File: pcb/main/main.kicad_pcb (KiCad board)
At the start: 2 copper layers, 77.5 x 78.7 mm, 43 parts, among them J1 USB_B, J2 USB_B, J3 RJ45, J4 RJ45, J5 STLink, J6 XH6, J7 Conn_01x05, J8 COLS, SW1 RST_SW, SW2 IS_LEFT, SW3 IS_LEFT, SW4 BOOT0_SW, SW5 BOOT1_SW, U1 LM1117-3.3, U2 STM32F103C8Tx, Y1 8MHz, Y2 32.768

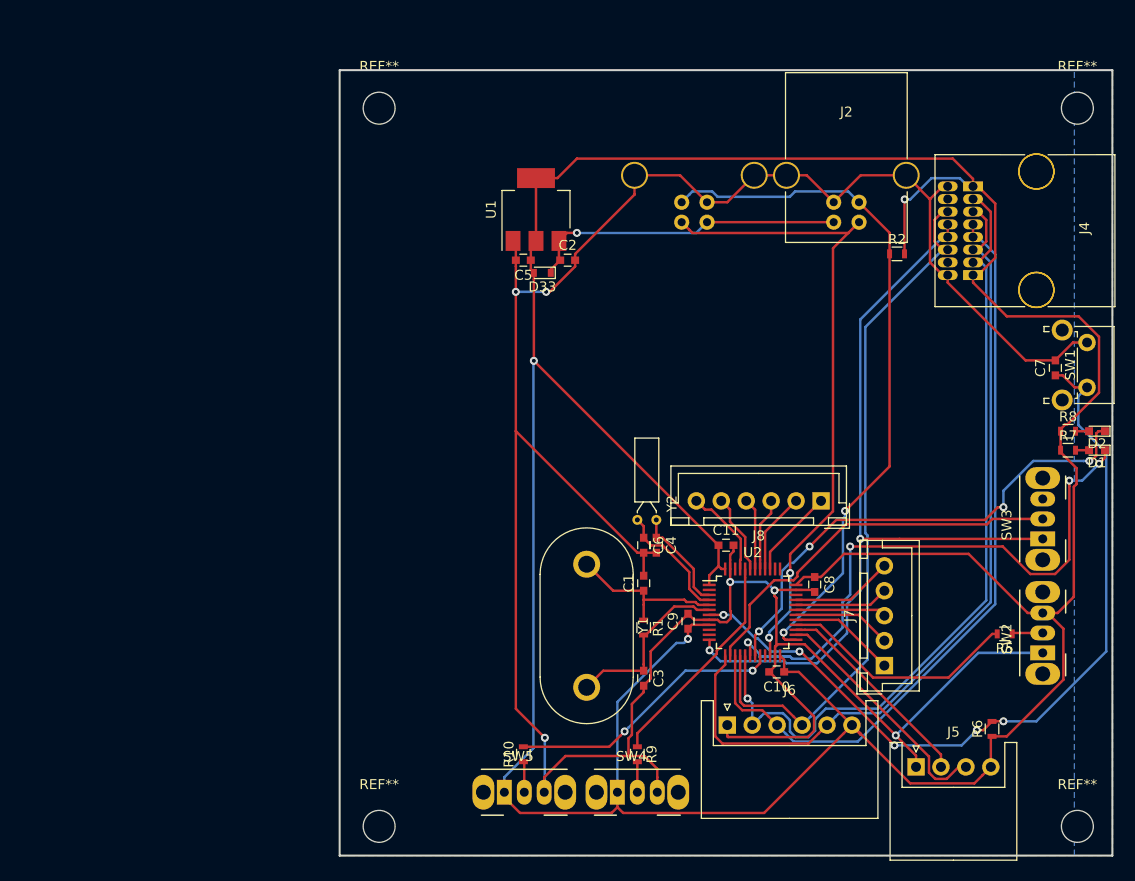
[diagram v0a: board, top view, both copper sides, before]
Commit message: fix main pcb
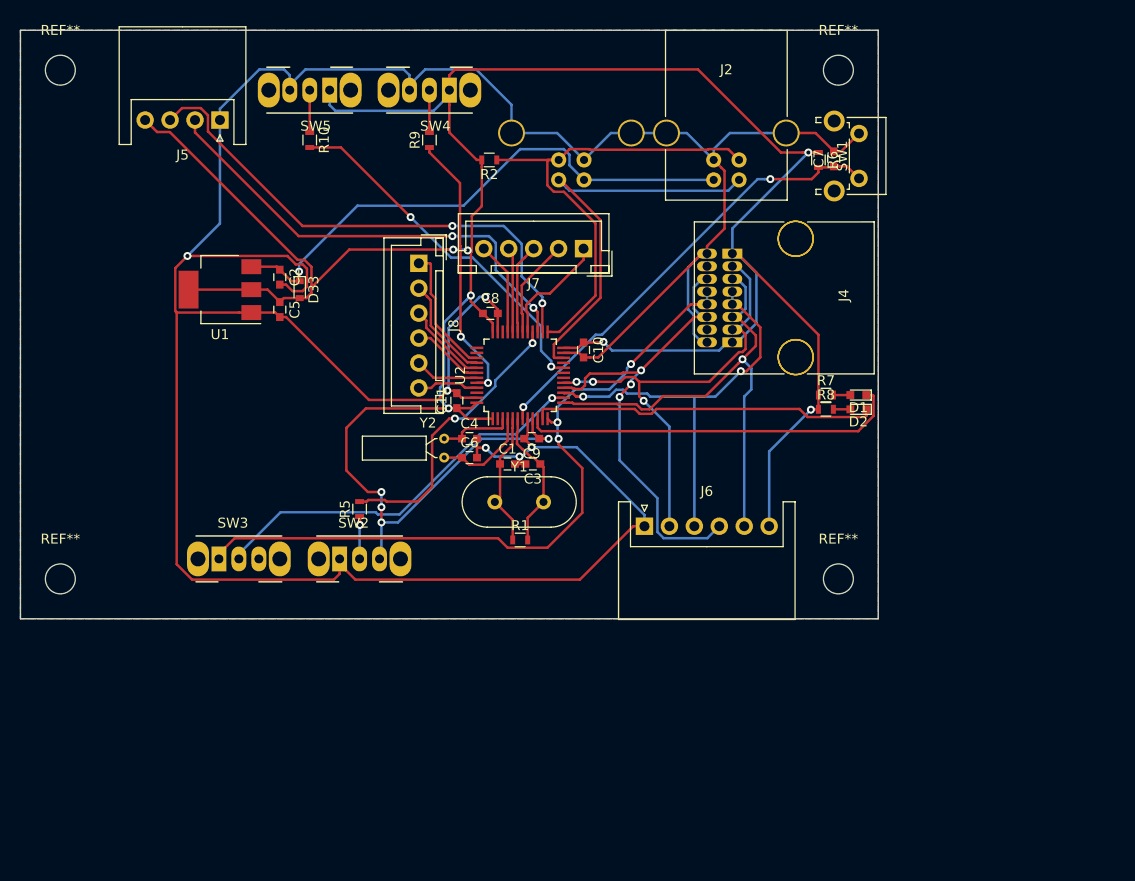
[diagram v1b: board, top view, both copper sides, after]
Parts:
- removed the REF** at (3.96, 3.81)
- removed the REF** at (74.0, 3.81)
- removed the REF** at (3.96, 75.8)
- removed the REF** at (74.0, 75.8)
- added REF**: MountingHole_3mm, Mounting_Holes:MountingHole_3mm, F.Cu at (-28.0, 0.00)
- added REF**: MountingHole_3mm, Mounting_Holes:MountingHole_3mm, F.Cu at (-28.0, 51.0)
- added REF**: MountingHole_3mm, Mounting_Holes:MountingHole_3mm, F.Cu at (50.0, 51.0)
- added REF**: MountingHole_3mm, Mounting_Holes:MountingHole_3mm, F.Cu at (50.0, 0.00)
- Y1: footprint Crystals:Crystal_HC33-U_Vertical -> Crystals:Crystal_HC49-4H_Vertical
- moved J5 95.3 mm to (-12.0, 5.00), turned to 180 degrees
- moved SW3 82.6 mm to (-12.1, 49.0), turned to 0 degrees
- moved SW5 72.5 mm to (-1.00, 2.00), turned to 180 degrees
- moved SW4 72.4 mm to (11.0, 2.00), turned to 180 degrees
- moved SW2 71.1 mm to (0.00, 49.0), turned to 0 degrees
- moved R5 65.9 mm to (2.00, 44.0), turned to 90 degrees
- moved R10 65.2 mm to (-3.00, 7.00), turned to 270 degrees
- moved R9 65.0 mm to (9.00, 7.00), turned to 90 degrees
- moved R6 59.6 mm to (48.0, 9.00), turned to 270 degrees
- moved J7 51.5 mm to (24.4, 17.9), turned to 180 degrees
- moved J8 46.8 mm to (7.94, 19.4), turned to 270 degrees
- moved C8 42.4 mm to (15.1, 24.4), turned to 0 degrees
- moved R2 42.0 mm to (15.0, 9.00), turned to 180 degrees
- moved C10 37.6 mm to (24.4, 28.1), turned to 270 degrees
- moved U2 33.3 mm to (18.1, 30.6), turned to 90 degrees
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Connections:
- U2 pad 10: Net-(U2-Pad10) -> /LED1
- U2 pad 11: Net-(U2-Pad11) -> /LED2
- U2 pad 18: /LED1 -> Net-(U2-Pad18)
- U2 pad 19: /LED2 -> Net-(U2-Pad19)
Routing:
- net +3V3: track 356.6 -> 287.0 mm, vias 3 -> 11
- net GND: track 280.5 -> 318.8 mm
- net /MOSI: track 82.5 -> 47.1 mm, vias 1 -> 3
- net /RST: track 80.8 -> 45.6 mm, vias 5 -> 2
- net /SS_T: track 84.1 -> 49.2 mm, vias 0 -> 1
- net /SCK: track 77.4 -> 43.1 mm, vias 0 -> 2
- net /SWDIO: track 24.5 -> 52.0 mm, vias 0 -> 2
- net /SWCLK: track 21.0 -> 46.6 mm, vias 0 -> 2
- net /LED1: track 61.8 -> 38.1 mm, vias 4 -> 0
- net +5V: track 32.0 -> 55.4 mm
- net /D-: track 64.4 -> 41.5 mm, vias 2 -> 0
- net /MISO: track 71.5 -> 48.9 mm, vias 0 -> 3
- net /D+: track 69.8 -> 48.8 mm, vias 2 -> 0
- net /LED2: track 50.1 -> 34.8 mm, vias 4 -> 0
- net /BOOT1: track 28.0 -> 36.4 mm
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- added copper zone on B.Cu, net (none)
- removed copper zone on B.Cu, net GND
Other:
- board size 77.5 x 78.7 mm -> 86 x 59 mm

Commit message: mechanical design
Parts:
- removed C1, C3: 20pF, Capacitors_SMD:C_0603
- removed C10, C11, C8, C9: 0.1uF, Capacitors_SMD:C_0603
- removed C2, C5, C7: 1uF, Capacitors_SMD:C_0603
- removed C4, C6: 12.5pF, Capacitors_SMD:C_0603
- removed D1: LED1, LEDs:LED_0603
- removed D2: LED2, LEDs:LED_0603
- removed D33: D, Diodes_SMD:D_0603
- removed J1, J2: USB_B, Connectors:USB_B
- removed J3, J4: RJ45, Connectors:RJ45_8
- removed J5: STLink, Connectors_JST:JST_XH_S04B-XH-A_04x2.50mm_Angled
- removed J6: XH6, Connectors_JST:JST_XH_S06B-XH-A_06x2.50mm_Angled
- removed J7: Conn_01x05, Connectors_JST:JST_XH_B05B-XH-A_05x2.50mm_Straight
- removed J8: COLS, Connectors_JST:JST_XH_B06B-XH-A_06x2.50mm_Straight
- removed R1: 10MΩ, Resistors_SMD:R_0603
- removed R10, R5, R6, R9: 4.7kΩ, Resistors_SMD:R_0603
- removed R2: 1.5kΩ, Resistors_SMD:R_0603
- removed R7, R8: R, Resistors_SMD:R_0603
- removed the REF** at (-28.0, 0.00)
- removed the REF** at (-28.0, 51.0)
- removed the REF** at (50.0, 51.0)
- removed the REF** at (50.0, 0.00)
- removed SW1: RST_SW, Buttons_Switches_THT:SW_Tactile_SPST_Angled_PTS645Vx31-2LFS
- removed SW2, SW3: IS_LEFT, Buttons_Switches_THT:SW_CuK_OS102011MA1QN1_SPDT_Angled
- removed SW4: BOOT0_SW, Buttons_Switches_THT:SW_CuK_OS102011MA1QN1_SPDT_Angled
- removed U1: LM1117-3.3, TO_SOT_Packages_SMD:SOT-223-3_TabPin2
- removed Y1: 8MHz, Crystals:Crystal_HC49-4H_Vertical
- removed Y2: 32.768, Crystals:Crystal_DS26_d2.0mm_l6.0mm_Horizontal
- added REF**: MountingHole_3.2mm_M3, MountingHole:MountingHole_3.2mm_M3, F.Cu at (132.7, 90.2)
- added REF**: MountingHole_3.2mm_M3, MountingHole:MountingHole_3.2mm_M3, F.Cu at (151.8, 147.3)
- added REF**: MountingHole_3.2mm_M3, MountingHole:MountingHole_3.2mm_M3, F.Cu at (132.7, 128.3)
- added REF**: MountingHole_3.2mm_M3, MountingHole:MountingHole_3.2mm_M3, F.Cu at (132.7, 147.3)
- added REF**: MountingHole_3.2mm_M3, MountingHole:MountingHole_3.2mm_M3, F.Cu at (132.7, 109.2)
- added REF**: MountingHole_3.2mm_M3, MountingHole:MountingHole_3.2mm_M3, F.Cu at (259.4, 147.3)
- added REF**: MountingHole_3.2mm_M3, MountingHole:MountingHole_3.2mm_M3, F.Cu at (259.4, 128.3)
- added REF**: MountingHole_3.2mm_M3, MountingHole:MountingHole_3.2mm_M3, F.Cu at (259.4, 109.2)
- added REF**: MountingHole_3.2mm_M3, MountingHole:MountingHole_3.2mm_M3, F.Cu at (221.3, 90.2)
- added SW10: K41, folivora:SW_Cherry_MX1A_1.00u_PCB, F.Cu at (133.3, 170.2)
- added SW15: K42, folivora:SW_Cherry_MX1A_1.00u_PCB, F.Cu at (156.2, 166.4)
- added SW20: K43, folivora:SW_Cherry_MX1A_1.00u_PCB, F.Cu at (179.1, 170.2)
- SW5: value BOOT1_SW -> K40; footprint Buttons_Switches_THT:SW_CuK_OS102011MA1QN1_SPDT_Angled -> folivora:SW_Cherry_MX1A_1.00u_PCB
- U2: value STM32F103C8Tx -> ADNS-9800; footprint Housings_QFP:LQFP-48_7x7mm_Pitch0.5mm -> folivora:ADNS-9800
- moved SW5 211.3 mm to (114.3, 179.1), turned to 30 degrees
- moved U2 180.3 mm to (141.0, 162.6)
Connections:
- SW5 pad 1: +3V3 -> /ROW4
- U2 pad 1: +3V3 -> Net-(C2-Pad1)
- U2 pad 10: /LED1 -> +3V3
- U2 pad 11: /LED2 -> GND
- U2 pad 12: /SS_K -> +3V3
- U2 pad 13: /SS_T -> Net-(U2-Pad13)
- U2 pad 14: Net-(SW3-Pad2) -> GND
- U2 pad 15: /SCK -> +3V3
- U2 pad 16: /MISO -> Net-(C2-Pad2)
- U2 pad 3: /XTAL_C -> /SS_Track
- U2 pad 4: /XTAL_D -> /MISO
- U2 pad 5: /XTAL_A -> /SCK
- U2 pad 6: /XTAL_B -> /MOSI
- U2 pad 7: /RST -> Net-(U2-Pad7)
- U2 pad 8: GND -> Net-(C2-Pad2)
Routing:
- net GND: track 318.8 -> 0.00 mm, vias 6 -> 0
- net +3V3: track 287.0 -> 0.00 mm, vias 11 -> 0
- net /SS_K: track 74.2 -> 0.00 mm, vias 3 -> 0
- net +5V: track 55.4 -> 0.00 mm, vias 1 -> 0
- net /SWDIO: track 52.0 -> 0.00 mm, vias 2 -> 0
- net /SS_T: track 49.2 -> 0.00 mm, vias 1 -> 0
- net /MISO: track 48.9 -> 0.00 mm, vias 3 -> 0
- net /D+: track 48.8 -> 0.00 mm
- net /MOSI: track 47.1 -> 0.00 mm, vias 3 -> 0
- net /SWCLK: track 46.6 -> 0.00 mm, vias 2 -> 0
- net /RST: track 45.6 -> 0.00 mm, vias 2 -> 0
- net /SCK: track 43.1 -> 0.00 mm, vias 2 -> 0
- net /D-: track 41.5 -> 0.00 mm
- net Net-(SW3-Pad2): track 39.7 -> 0.00 mm, vias 1 -> 0
- net /LED1: track 38.1 -> 0.00 mm
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- removed copper zone on B.Cu, net (none)
- removed copper zone on F.Cu, net GND
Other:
- board size 86 x 59 mm -> 163.2 x 107.3 mm
